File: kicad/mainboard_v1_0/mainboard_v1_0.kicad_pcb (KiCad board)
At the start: 2 copper layers, 133.8 x 99.2 mm, 36 parts, among them J1 Conn_01x02, J2 Conn_01x06, J3 Conn_01x04, J4 Conn_01x04, J5 Conn_01x05, J6 Conn_01x08, SW1 SW_DIP_x06, U1 stm32f4_disco_board, U2 74HC245, U3 LM2596_MODULE, U4 AMS1117-3.3, U5 AMS1117-5.0

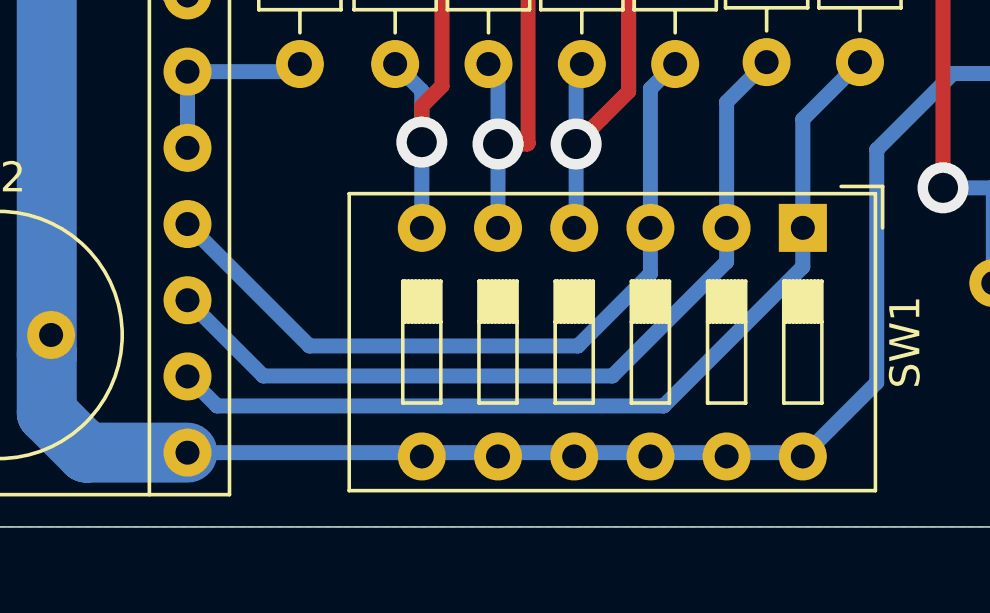
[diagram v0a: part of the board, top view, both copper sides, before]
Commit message: fix hardware
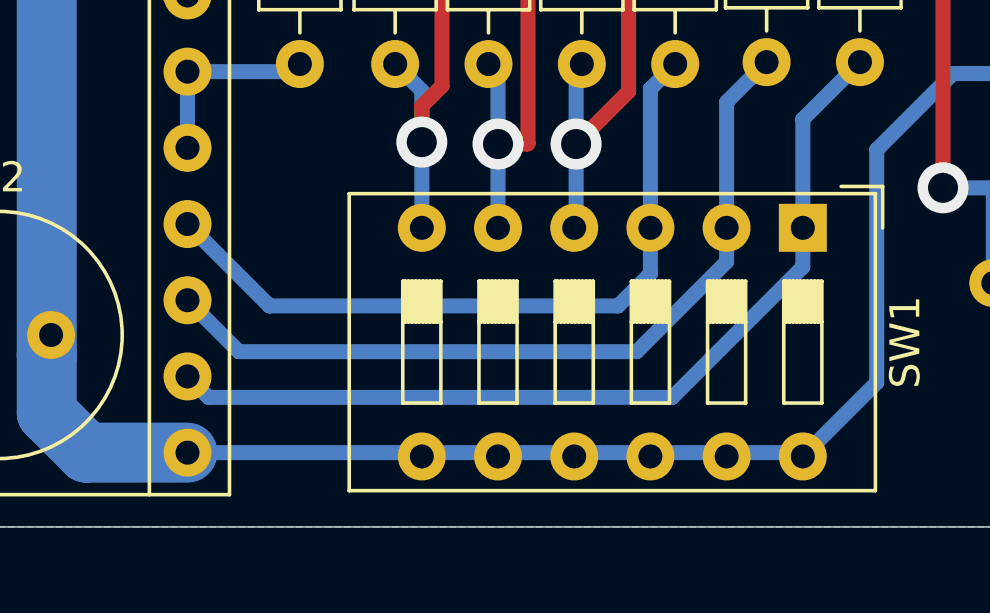
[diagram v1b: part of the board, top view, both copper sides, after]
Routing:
- net A4988_1_MS3: track 25.4 -> 24.3 mm
- net A4988_1_MS2: track 27.8 -> 27.1 mm
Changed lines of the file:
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@@
   )
   (setup
-    (last_trace_width 0.5)
+    (last_trace_width 0.6)
     (user_trace_width 0.5)
     (user_trace_width 1)
@@
     (visible_elements FFFFFF7F)
     (pcbplotparams
-      (layerselection 0x010fc_ffffffff)
+      (layerselection 0x01000_ffffffff)
       (usegerberextensions false)
       (usegerberattributes false)
@@
       (padsonsilk false)
       (subtractmaskfromsilk false)
-      (outputformat 1)
+      (outputformat 4)
       (mirror false)
-      (drillshape 1)
+      (drillshape 2)
       (scaleselection 1)
-      (outputdirectory ""))
+      (outputdirectory "../../../../Desktop/"))
   )
   (net 0 "")
@@
   (segment (start 20.3835 127.8255) (end 29.6545 127.8255) (width 0.5) (layer B.Cu) (net 6))
   (segment (start 20.3835 125.2855) (end 29.6545 125.2855) (width 0.5) (layer B.Cu) (net 7))
-  (segment (start 55.372 129.3495) (end 57.785 126.9365) (width 0.5) (layer B.Cu) (net 8))
-  (segment (start 46.4185 129.3495) (end 55.372 129.3495) (width 0.5) (layer B.Cu) (net 8))
-  (segment (start 57.785 126.9365) (end 57.785 125.4125) (width 0.5) (layer B.Cu) (net 8))
-  (segment (start 42.3545 125.2855) (end 46.4185 129.3495) (width 0.5) (layer B.Cu) (net 8))
   (segment (start 57.785 120.777) (end 57.785 125.4125) (width 0.5) (layer B.Cu) (net 8))
   (segment (start 58.6105 119.9515) (end 57.785 120.777) (width 0.5) (layer B.Cu) (net 8))
+  (segment (start 57.785 126.9365) (end 57.785 125.4125) (width 0.5) (layer B.Cu) (net 8))
+  (segment (start 56.7055 128.016) (end 57.785 126.9365) (width 0.5) (layer B.Cu) (net 8))
+  (segment (start 42.3545 125.2855) (end 45.085 128.016) (width 0.5) (layer B.Cu) (net 8))
+  (segment (start 45.085 128.016) (end 56.7055 128.016) (width 0.5) (layer B.Cu) (net 8))
   (segment (start 20.3835 122.7455) (end 29.6545 122.7455) (width 0.5) (layer B.Cu) (net 9))
-  (segment (start 42.3545 127.8255) (end 44.878511 130.349511) (width 0.5) (layer B.Cu) (net 10))
-  (segment (start 44.878511 130.349511) (end 56.519359 130.349511) (width 0.5) (layer B.Cu) (net 10))
-  (segment (start 60.325 126.54387) (end 60.325 125.4125) (width 0.5) (layer B.Cu) (net 10))
-  (segment (start 56.519359 130.349511) (end 60.325 126.54387) (width 0.5) (layer B.Cu) (net 10))
   (segment (start 60.325 121.2215) (end 60.325 125.4125) (width 0.5) (layer B.Cu) (net 10))
   (segment (start 61.6585 119.888) (end 60.325 121.2215) (width 0.5) (layer B.Cu) (net 10))
+  (segment (start 60.325 126.54387) (end 60.325 125.4125) (width 0.5) (layer B.Cu) (net 10))
+  (segment (start 57.32887 129.54) (end 60.325 126.54387) (width 0.5) (layer B.Cu) (net 10))
+  (segment (start 42.3545 127.8255) (end 44.069 129.54) (width 0.5) (layer B.Cu) (net 10))
+  (segment (start 44.069 129.54) (end 57.32887 129.54) (width 0.5) (layer B.Cu) (net 10))
   (segment (start 20.3835 120.2055) (end 29.6545 120.2055) (width 0.5) (layer B.Cu) (net 11))
-  (segment (start 58.227978 131.349522) (end 62.865 126.7125) (width 0.5) (layer B.Cu) (net 12))
-  (segment (start 43.338522 131.349522) (end 58.227978 131.349522) (width 0.5) (layer B.Cu) (net 12))
-  (segment (start 42.3545 130.3655) (end 43.338522 131.349522) (width 0.5) (layer B.Cu) (net 12))
-  (segment (start 62.865 126.7125) (end 62.865 125.4125) (width 0.5) (layer B.Cu) (net 12))
   (segment (start 62.865 121.793) (end 62.865 125.4125) (width 0.5) (layer B.Cu) (net 12))
   (segment (start 64.77 119.888) (end 62.865 121.793) (width 0.5) (layer B.Cu) (net 12))
+  (segment (start 62.865 126.7125) (end 62.865 125.4125) (width 0.5) (layer B.Cu) (net 12))
+  (segment (start 58.5135 131.064) (end 62.865 126.7125) (width 0.5) (layer B.Cu) (net 12))
+  (segment (start 42.3545 130.3655) (end 43.053 131.064) (width 0.5) (layer B.Cu) (net 12))
+  (segment (start 43.053 131.064) (end 58.5135 131.064) (width 0.5) (layer B.Cu) (net 12))
   (segment (start 29.053 117.064) (end 29.6545 117.6655) (width 0.5) (layer B.Cu) (net 13))
   (segment (start 26.035 117.064) (end 29.053 117.064) (width 0.5) (layer B.Cu) (net 13))
